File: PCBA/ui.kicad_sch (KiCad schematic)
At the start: 6 parts, among them J701 FH12-24S-0.5SH(55), Q701 2N7002, SW801 SW_Push, SW802 SW_Push, SW803 SW_Push

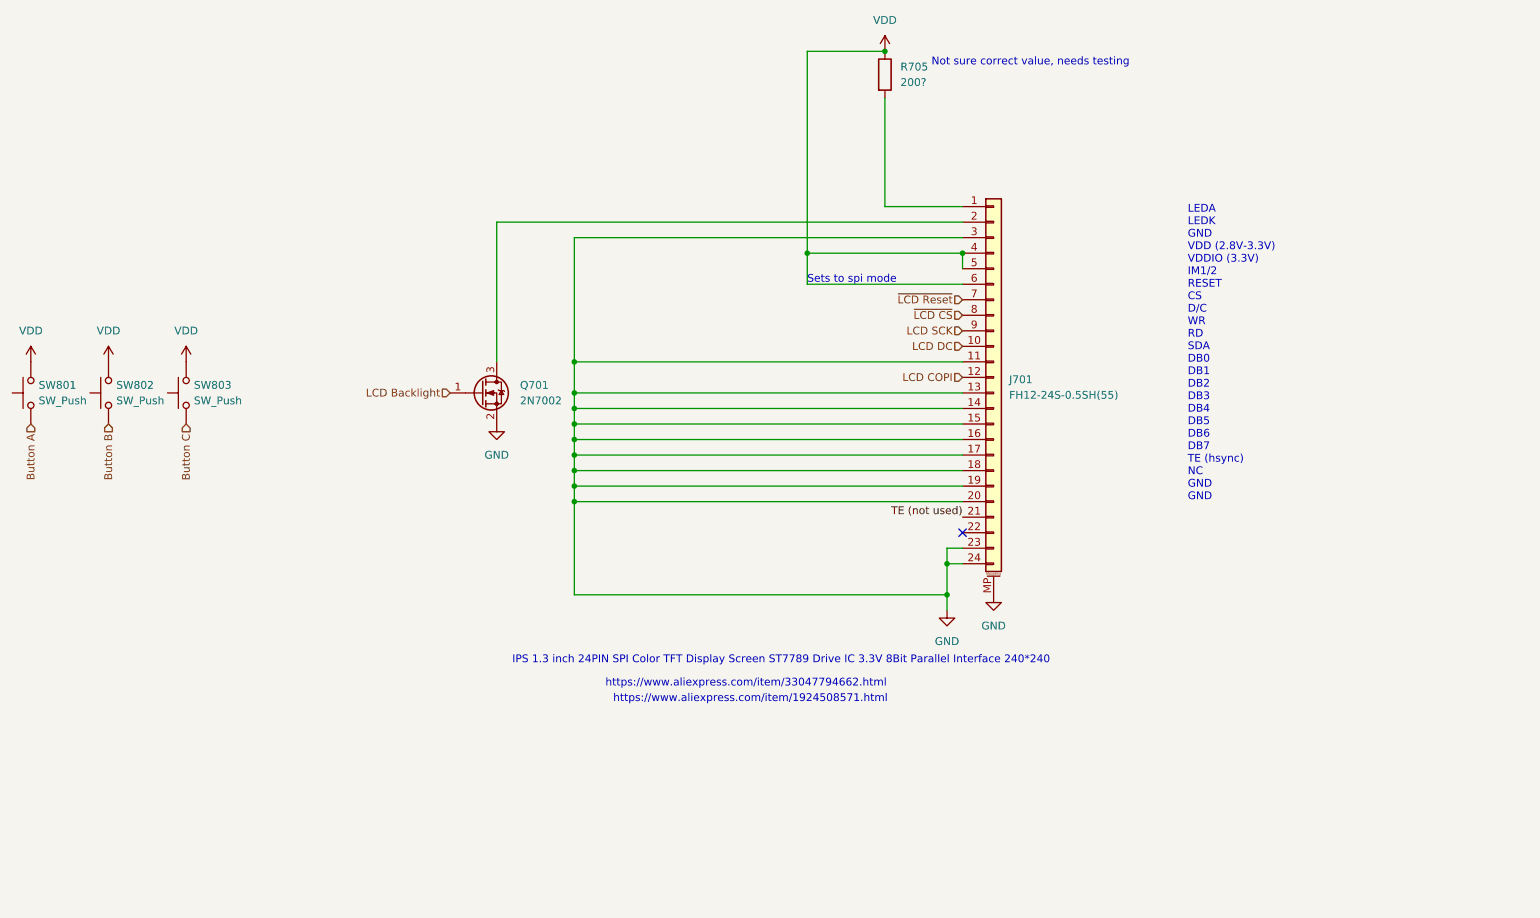
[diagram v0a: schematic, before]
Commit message: Rough outline
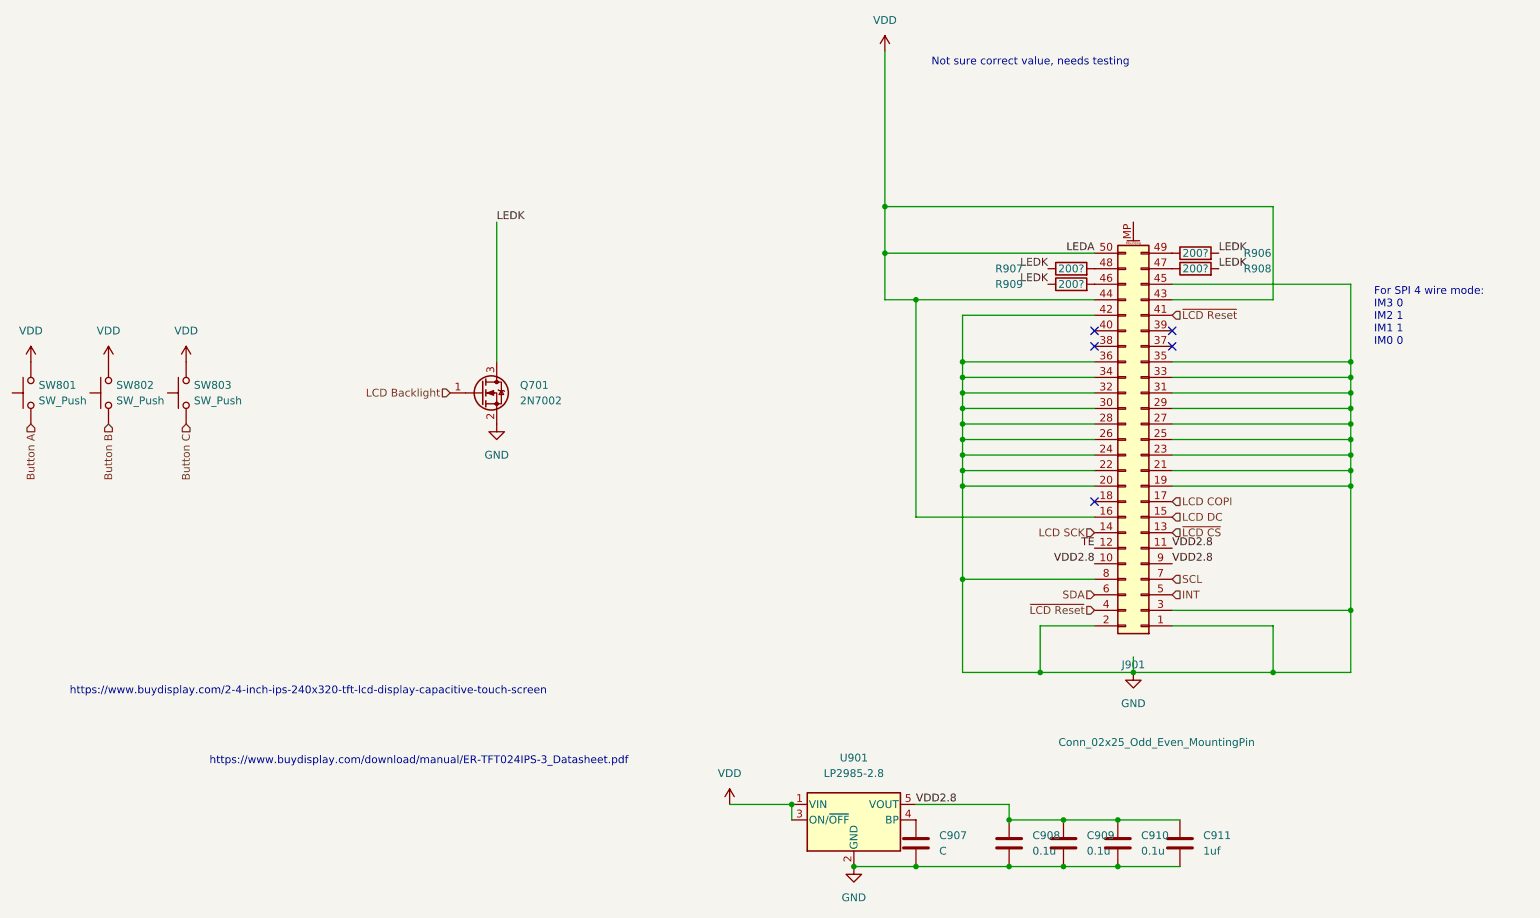
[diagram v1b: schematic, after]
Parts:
- removed J701: FH12-24S-0.5SH(55), Connector_FFC-FPC:Hirose_FH12-24S-0.5SH_1x24-1MP_P0.50mm_Horizontal, symbol Connector_Generic_MountingPin:Conn_01x24_MountingPin
- removed R705: 200?, Resistor_SMD:R_0603_1608Metric, symbol Device:R
- added C907: C, Capacitor_SMD:C_0603_1608Metric, symbol Device:C
- added C908, C909, C910: 0.1u, Capacitor_SMD:C_0603_1608Metric, symbol Device:C
- added C911: 1uf, Capacitor_SMD:C_0603_1608Metric, symbol Device:C
- added J901: Conn_02x25_Odd_Even_MountingPin, Connector_FFC-FPC:Molex_54132-5033_1x50-1MP_P0.5mm_Horizontal, symbol Connector_Generic_MountingPin:Conn_02x25_Odd_Even_MountingPin
- added R906, R907, R908, R909: 200?, Resistor_SMD:R_0603_1608Metric, symbol Device:R
- added U901: LP2985-2.8, Package_TO_SOT_SMD:SOT-23-5, symbol Regulator_Linear:LP2985-2.8
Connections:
- net GND: now also C907.2, C908.2, C909.2, C910.2, C911.2, J901.1 (Pin_1), J901.19 (Pin_19), J901.2 (Pin_2), J901.20 (Pin_20), J901.21 (Pin_21), J901.22 (Pin_22), J901.23 (Pin_23), J901.24 (Pin_24), J901.25 (Pin_25), J901.26 (Pin_26), J901.27 (Pin_27), J901.28 (Pin_28), J901.29 (Pin_29), J901.3 (Pin_3), J901.30 (Pin_30), J901.31 (Pin_31), J901.32 (Pin_32), J901.33 (Pin_33), J901.34 (Pin_34), J901.35 (Pin_35), J901.36 (Pin_36), J901.42 (Pin_42), J901.45 (Pin_45), J901.8 (Pin_8), U901.2 (GND)
- net LCD COPI: now also J901.17 (Pin_17)
- net LCD DC: now also J901.15 (Pin_15)
- net LCD SCK: now also J901.14 (Pin_14)
- net VDD: now also J901.16 (Pin_16), J901.43 (Pin_43), J901.44 (Pin_44), J901.50 (Pin_50), U901.1 (VIN), U901.3 (ON/~{OFF})
- net ~{LCD CS}: now also J901.13 (Pin_13)
- net ~{LCD Reset}: now also J901.4 (Pin_4), J901.41 (Pin_41)
- net LEDK: now reaches Q701.3 (D)
- net LEDK: now also R906.2, R907.1, R908.2, R909.1
- new net: J901.48 (Pin_48), R907.2
- new net: C907.1, U901.4 (BP)
- new net: J901.46 (Pin_46), R909.2
- new net: J901.47 (Pin_47), R908.1
- new net: J901.49 (Pin_49), R906.1
- new net INT: J901.5 (Pin_5)
- new net SCL: J901.7 (Pin_7)
- new net SDA: J901.6 (Pin_6)
- new net TE: J901.12 (Pin_12)
- new net VDD2.8: C908.1, C909.1, C910.1, C911.1, J901.10 (Pin_10), J901.11 (Pin_11), J901.9 (Pin_9), U901.5 (VOUT)
- no-connect marks 1 -> 5
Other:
- note added: "For SPI 4 wire mode: IM3 0 IM2 1 IM1 1 IM0 0"
- note added: "https://www.buydisplay.com/2-4-inch-ips-240x320-tft-lcd-display-capacitive-touch-screen"
- note added: "https://www.buydisplay.com/download/manual/ER-TFT024IPS-3_Datasheet.pdf"
- note removed: "IPS 1.3 inch 24PIN SPI Color TFT Display Screen ST7789 Drive IC 3.3V 8Bit Parallel Interface 240*240"
- note removed: "LEDA LEDK GND VDD (2.8V-3.3V) VDDIO (3.3V) IM1/2 RESET CS D/C WR RD SDA DB0 DB1 DB2 DB3 DB4 DB5 DB6 DB7 TE (hsync) NC GND GND"
- note removed: "Sets to spi mode"
- note removed: "https://www.aliexpress.com/item/1924508571.html"
- note removed: "https://www.aliexpress.com/item/33047794662.html"
